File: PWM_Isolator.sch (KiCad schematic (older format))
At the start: 12 parts, among them P1 PWM_OUT_1, P10 PWM_OUT_2, P2 PWR_Jumper1, P3 Motor_Pwr1, P4 GND_IN_1, P5 Pololu PWM + Power rail, P6 NC, P7 GND_IN_2, P8 PWR_Jumper2, P9 Motor_Pwr2, U1 Si8660BA-B-IS1, U2 Si8660BA-B-IS1

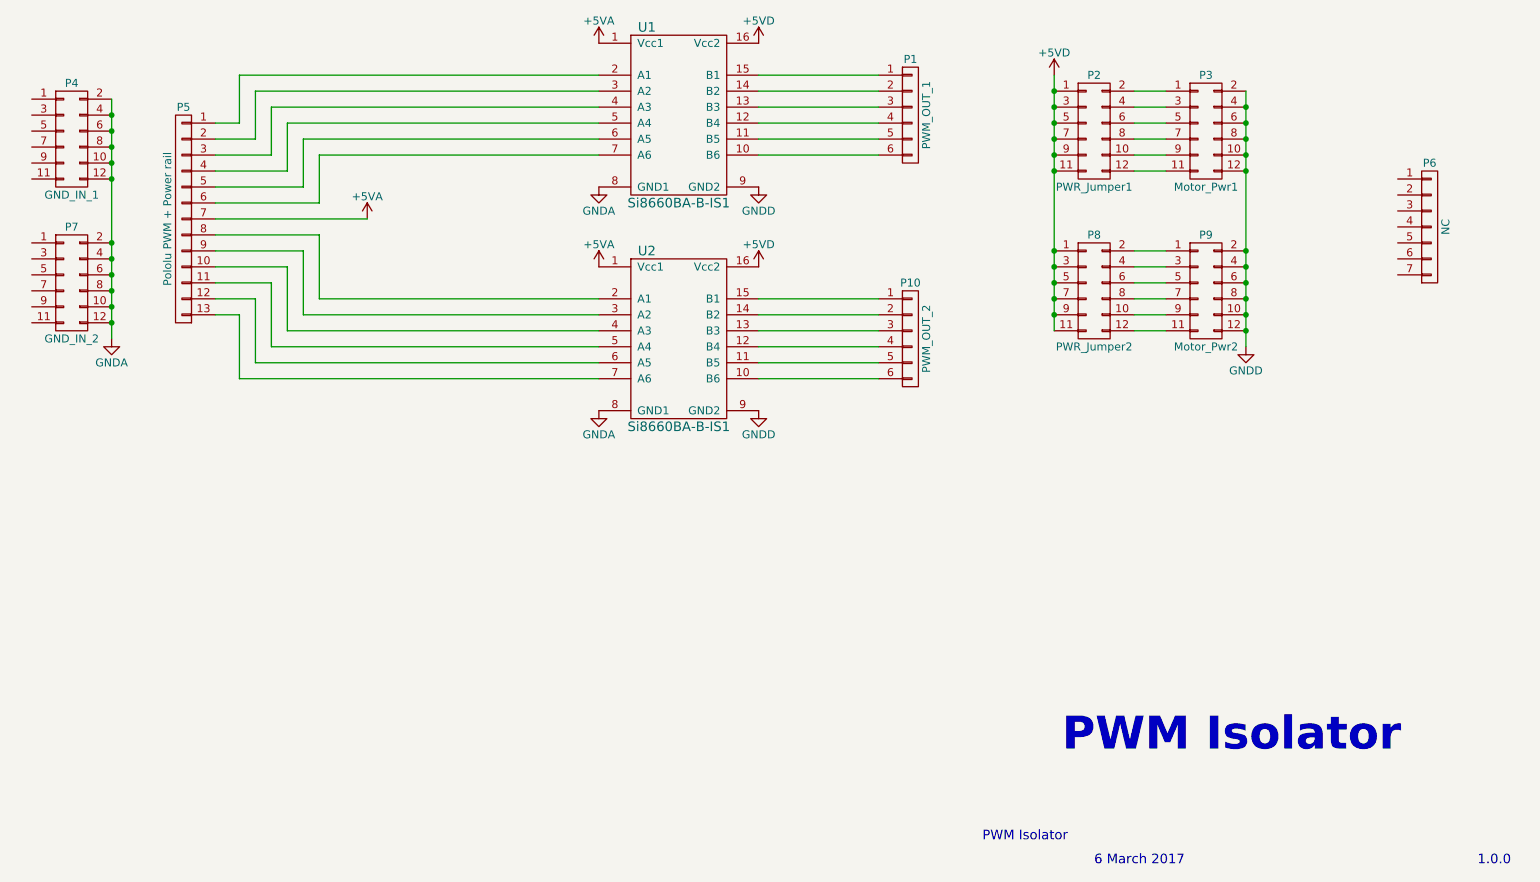
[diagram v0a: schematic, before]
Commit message: Finished with PCB and Net
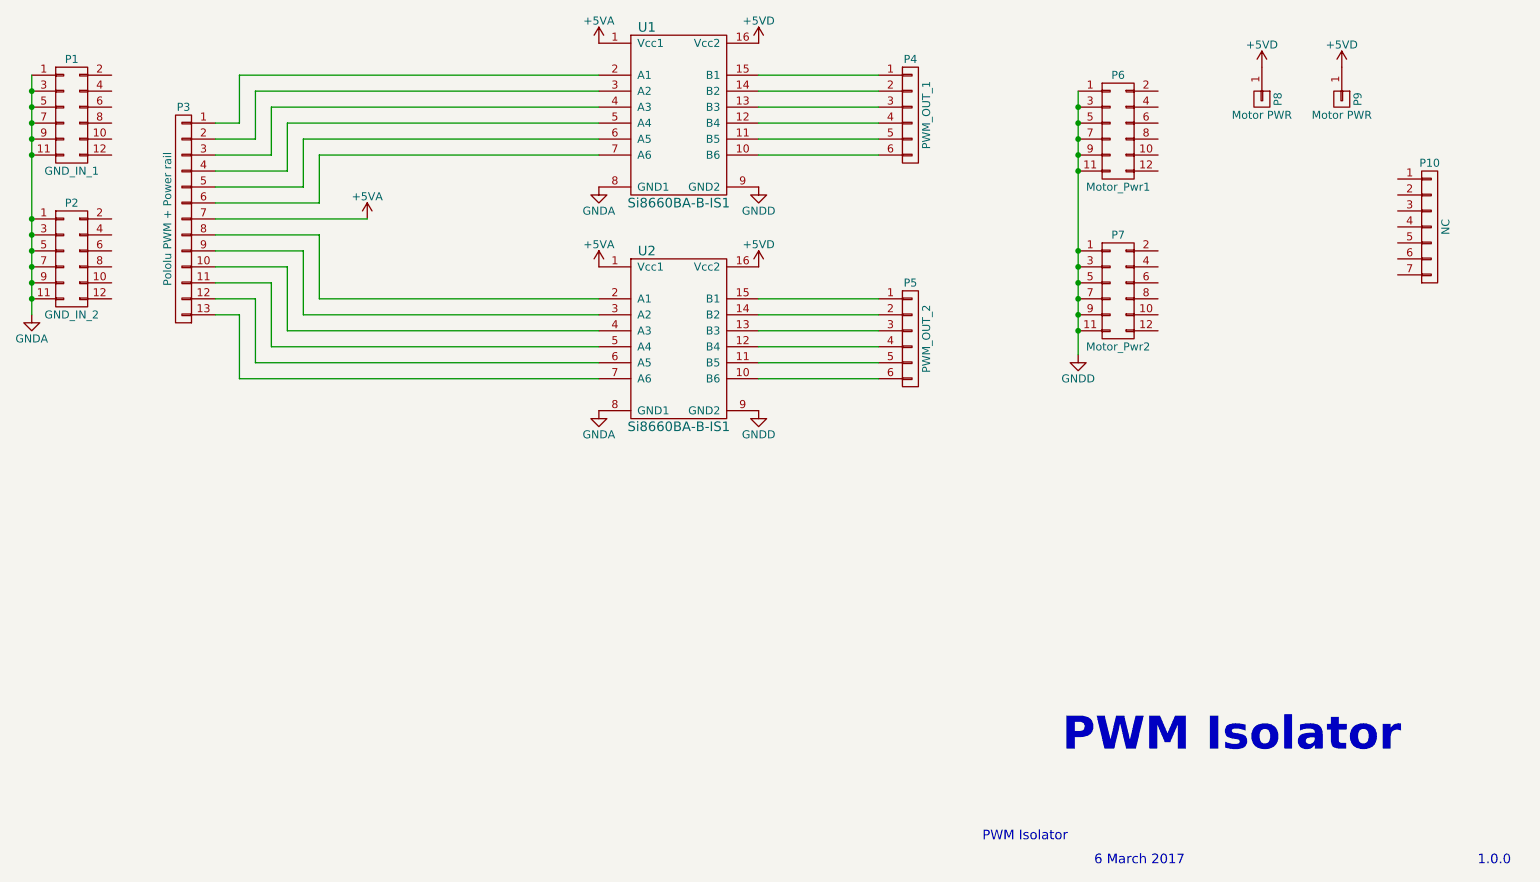
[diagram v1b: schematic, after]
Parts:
- removed P2: PWR_Jumper1, Pin_Headers:Pin_Header_Straight_SMT_02x06, symbol CONN_02X06
- removed P8: PWR_Jumper2, Pin_Headers:Pin_Header_Straight_SMT_02x06, symbol CONN_02X06
- added P8, P9: Motor PWR, Pin_Headers:Pin_Header_Straight_1x01, symbol CONN_01X01
- renumbered P4 to P1, P6 to P10, P7 to P2, P5 to P3, P1 to P4, P10 to P5, P3 to P6, P9 to P7
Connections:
- net +5VD: now also P8.1 (P1), P9.1 (P1)
- net GNDA: now also P1.1 (P1), P1.11 (P11), P1.3 (P3), P1.5 (P5), P1.7 (P7), P1.9 (P9), P2.1 (P1), P2.11 (P11), P2.3 (P3), P2.5 (P5), P2.7 (P7), P2.9 (P9); no longer P1.10 (P10), P1.12 (P12), P1.2 (P2), P1.4 (P4), P1.6 (P6), P1.8 (P8), P2.10 (P10), P2.12 (P12), P2.2 (P2), P2.4 (P4), P2.6 (P6), P2.8 (P8)
- net GNDD: now also P6.1 (P1), P6.11 (P11), P6.3 (P3), P6.5 (P5), P6.7 (P7), P6.9 (P9), P7.1 (P1), P7.11 (P11), P7.3 (P3), P7.5 (P5), P7.7 (P7), P7.9 (P9); no longer P6.10 (P10), P6.12 (P12), P6.2 (P2), P6.4 (P4), P6.6 (P6), P6.8 (P8), P7.10 (P10), P7.12 (P12), P7.2 (P2), P7.4 (P4), P7.6 (P6), P7.8 (P8)
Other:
- moved on the sheet: P1, P2, P6, P7
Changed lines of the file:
@@
 LIBS:valves
 LIBS:zeabus
+LIBS:PWM_Isolator-cache
 EELAYER 25 0
 EELAYER END
@@
 $EndComp
 $Comp
-L CONN_01X13 P5
+L CONN_01X13 P3
 U 1 1 58BD71B6
 P 2550 3600
-F 0 "P5" H 2550 4300 50  0000 C CNN
+F 0 "P3" H 2550 4300 50  0000 C CNN
 F 1 "Pololu PWM + Power rail" V 2650 3600 50  0000 C CNN
 F 2 "Socket_Strips:Socket_Strip_Straight_1x13" H 2550 3600 50  0001 C CNN
@@
 $EndComp
 $Comp
-L CONN_02X06 P7
+L CONN_02X06 P2
 U 1 1 58BD71DC
-P 1850 4000
-F 0 "P7" H 1850 4350 50  0000 C CNN
-F 1 "GND_IN_2" H 1850 3650 50  0000 C CNN
-F 2 "Socket_Strips:Socket_Strip_Straight_2x06" H 1850 2800 50  0001 C CNN
-F 3 "" H 1850 2800 50  0000 C CNN
-	1    1850 4000
-	1    0    0    -1
-$EndComp
-$Comp
-L CONN_01X07 P6
+P 1850 3850
+F 0 "P2" H 1850 4200 50  0000 C CNN
+F 1 "GND_IN_2" H 1850 3500 50  0000 C CNN
+F 2 "Socket_Strips:Socket_Strip_Straight_2x06" H 1850 2650 50  0001 C CNN
+F 3 "" H 1850 2650 50  0000 C CNN
+	1    1850 3850
+	1    0    0    -1
+$EndComp
+$Comp
+L CONN_01X07 P10
 U 1 1 58BD7246
 P 10350 3650
-F 0 "P6" H 10350 4050 50  0000 C CNN
+F 0 "P10" H 10350 4050 50  0000 C CNN
 F 1 "NC" V 10450 3650 50  0000 C CNN
 F 2 "Socket_Strips:Socket_Strip_Straight_1x07" H 10350 3650 50  0001 C CNN
@@
 $EndComp
 $Comp
-L CONN_02X06 P4
+L CONN_02X06 P1
 U 1 1 58BD72FA
-P 1850 3100
-F 0 "P4" H 1850 3450 50  0000 C CNN
-F 1 "GND_IN_1" H 1850 2750 50  0000 C CNN
-F 2 "Socket_Strips:Socket_Strip_Straight_2x06" H 1850 1900 50  0001 C CNN
-F 3 "" H 1850 1900 50  0000 C CNN
-	1    1850 3100
-	1    0    0    -1
-$EndComp
-$Comp
-L CONN_02X06 P3
+P 1850 2950
+F 0 "P1" H 1850 3300 50  0000 C CNN
+F 1 "GND_IN_1" H 1850 2600 50  0000 C CNN
+F 2 "Socket_Strips:Socket_Strip_Straight_2x06" H 1850 1750 50  0001 C CNN
+F 3 "" H 1850 1750 50  0000 C CNN
+	1    1850 2950
+	1    0    0    -1
+$EndComp
+$Comp
+L CONN_02X06 P6
 U 1 1 58BD7333
-P 8950 3050
-F 0 "P3" H 8950 3400 50  0000 C CNN
-F 1 "Motor_Pwr1" H 8950 2700 50  0000 C CNN
-F 2 "Pin_Headers:Pin_Header_Straight_2x06" H 8950 1850 50  0001 C CNN
-F 3 "" H 8950 1850 50  0000 C CNN
-	1    8950 3050
-	1    0    0    -1
-$EndComp
-$Comp
-L CONN_02X06 P2
-U 1 1 58BD7377
-P 8250 3050
-F 0 "P2" H 8250 3400 50  0000 C CNN
-F 1 "PWR_Jumper1" H 8250 2700 50  0000 C CNN
-F 2 "Pin_Headers:Pin_Header_Straight_SMT_02x06" H 8250 1850 50  0001 C CNN
-F 3 "" H 8250 1850 50  0000 C CNN
-	1    8250 3050
-	1    0    0    -1
-$EndComp
-$Comp
-L CONN_01X06 P1
+P 8400 3050
+F 0 "P6" H 8400 3400 50  0000 C CNN
+F 1 "Motor_Pwr1" H 8400 2700 50  0000 C CNN
+F 2 "Pin_Headers:Pin_Header_Straight_2x06" H 8400 1850 50  0001 C CNN
+F 3 "" H 8400 1850 50  0000 C CNN
+	1    8400 3050
+	1    0    0    -1
+$EndComp
+$Comp
+L CONN_01X06 P4
 U 1 1 58BD73C1
 P 7100 2950
-F 0 "P1" H 7100 3300 50  0000 C CNN
+F 0 "P4" H 7100 3300 50  0000 C CNN
 F 1 "PWM_OUT_1" V 7200 2950 50  0000 C CNN
 F 2 "Pin_Headers:Pin_Header_Straight_1x06" H 7100 2950 50  0001 C CNN
@@
 $EndComp
 $Comp
-L CONN_01X06 P10
+L CONN_01X06 P5
 U 1 1 58BD7462
 P 7100 4350
-F 0 "P10" H 7100 4700 50  0000 C CNN
+F 0 "P5" H 7100 4700 50  0000 C CNN
 F 1 "PWM_OUT_2" V 7200 4350 50  0000 C CNN
 F 2 "Pin_Headers:Pin_Header_Straight_1x06" H 7100 4350 50  0001 C CNN
@@
 $EndComp
 $Comp
-L CONN_02X06 P8
-U 1 1 58BD749E
-P 8250 4050
-F 0 "P8" H 8250 4400 50  0000 C CNN
-F 1 "PWR_Jumper2" H 8250 3700 50  0000 C CNN
-F 2 "Pin_Headers:Pin_Header_Straight_SMT_02x06" H 8250 2850 50  0001 C CNN
-F 3 "" H 8250 2850 50  0000 C CNN
-	1    8250 4050
-	1    0    0    -1
-$EndComp
-$Comp
-L CONN_02X06 P9
+L CONN_02X06 P7
 U 1 1 58BD7515
-P 8950 4050
-F 0 "P9" H 8950 4400 50  0000 C CNN
-F 1 "Motor_Pwr2" H 8950 3700 50  0000 C CNN
-F 2 "Pin_Headers:Pin_Header_Straight_2x06" H 8950 2850 50  0001 C CNN
-F 3 "" H 8950 2850 50  0000 C CNN
-	1    8950 4050
-	1    0    0    -1
-$EndComp
-Wire Wire Line
-	2100 2850 2100 4350
-Connection ~ 2100 2950
-Connection ~ 2100 3050
-Connection ~ 2100 3150
-Connection ~ 2100 3250
-Connection ~ 2100 3350
-Connection ~ 2100 3750
-Connection ~ 2100 3850
-Connection ~ 2100 3950
-Connection ~ 2100 4050
-Connection ~ 2100 4150
+P 8400 4050
+F 0 "P7" H 8400 4400 50  0000 C CNN
+F 1 "Motor_Pwr2" H 8400 3700 50  0000 C CNN
+F 2 "Pin_Headers:Pin_Header_Straight_2x06" H 8400 2850 50  0001 C CNN
+F 3 "" H 8400 2850 50  0000 C CNN
+	1    8400 4050
+	1    0    0    -1
+$EndComp
 $Comp
 L GNDA #PWR01
 U 1 1 58BD7AF0
-P 2100 4350
-F 0 "#PWR01" H 2100 4100 50  0001 C CNN
-F 1 "GNDA" H 2100 4200 50  0000 C CNN
-F 2 "" H 2100 4350 50  0000 C CNN
-F 3 "" H 2100 4350 50  0000 C CNN
-	1    2100 4350
+P 1600 4200
+F 0 "#PWR01" H 1600 3950 50  0001 C CNN
+F 1 "GNDA" H 1600 4050 50  0000 C CNN
+F 2 "" H 1600 4200 50  0000 C CNN
+F 3 "" H 1600 4200 50  0000 C CNN
+	1    1600 4200
 	1    0    0    -1
 $EndComp
@@
 	1    0    0    -1
 $EndComp
-Connection ~ 2100 4250
 Wire Wire Line
 	2750 3000 2900 3000
@@
 L +5VD #PWR04
 U 1 1 58BD81D8
-P 8000 2700
-F 0 "#PWR04" H 8000 2550 50  0001 C CNN
-F 1 "+5VD" H 8000 2840 50  0000 C CNN
-F 2 "" H 8000 2700 50  0000 C CNN
-F 3 "" H 8000 2700 50  0000 C CNN
-	1    8000 2700
+P 9300 2650
+F 0 "#PWR04" H 9300 2500 50  0001 C CNN
+F 1 "+5VD" H 9300 2790 50  0000 C CNN
+F 2 "" H 9300 2650 50  0000 C CNN
+F 3 "" H 9300 2650 50  0000 C CNN
+	1    9300 2650
 	1    0    0    -1
 $EndComp
@@
 Wire Wire Line
 	6150 4600 6900 4600
-Wire Wire Line
-	8500 2800 8700 2800
-Wire Wire Line
-	8700 2900 8500 2900
-Wire Wire Line
-	8500 3000 8700 3000
-Wire Wire Line
-	8700 3100 8500 3100
-Wire Wire Line
-	8500 3200 8700 3200
-Wire Wire Line
-	8700 3300 8500 3300
-Wire Wire Line
-	8500 3800 8700 3800
-Wire Wire Line
-	8700 3900 8500 3900
-Wire Wire Line
-	8700 4000 8500 4000
-Wire Wire Line
-	8500 4100 8700 4100
-Wire Wire Line
-	8700 4200 8500 4200
-Wire Wire Line
-	8500 4300 8700 4300
-Wire Wire Line
-	9200 2800 9200 4400
-Connection ~ 9200 4200
-Connection ~ 9200 4100
-Connection ~ 9200 4000
-Connection ~ 9200 3900
-Connection ~ 9200 3800
-Connection ~ 9200 3300
-Connection ~ 9200 3200
-Connection ~ 9200 3100
-Connection ~ 9200 3000
-Connection ~ 9200 2900
 $Comp
 L GNDD #PWR07
 U 1 1 58BD98A2
-P 9200 4400
-F 0 "#PWR07" H 9200 4150 50  0001 C CNN
-F 1 "GNDD" H 9200 4250 50  0000 C CNN
-F 2 "" H 9200 4400 50  0000 C CNN
-F 3 "" H 9200 4400 50  0000 C CNN
-	1    9200 4400
+P 8150 4450
+F 0 "#PWR07" H 8150 4200 50  0001 C CNN
+F 1 "GNDD" H 8150 4300 50  0000 C CNN
+F 2 "" H 8150 4450 50  0000 C CNN
+F 3 "" H 8150 4450 50  0000 C CNN
+	1    8150 4450
 	1    0    0    -1
 $EndComp
@@
 	1    0    0    -1
 $EndComp
-Connection ~ 9200 4300
-Wire Wire Line
-	8000 2700 8000 4300
-Connection ~ 8000 4200
-Connection ~ 8000 4100
-Connection ~ 8000 4000
-Connection ~ 8000 3900
-Connection ~ 8000 3800
-Connection ~ 8000 3300
-Connection ~ 8000 3200
-Connection ~ 8000 3100
-Connection ~ 8000 3000
-Connection ~ 8000 2900
 $Comp
 L +5VA #PWR010
@@
 	1    0    0    -1
 $EndComp
-Connection ~ 8000 2800
 Text Notes 8050 6950 0    206  ~ 41
 PWM Isolator\n
@@
 Text Notes 7550 7500 0    60   ~ 0
 PWM Isolator\n
+Wire Wire Line
+	1600 2700 1600 4200
+Connection ~ 1600 2800
+Connection ~ 1600 2900
+Connection ~ 1600 3000
+Connection ~ 1600 3100
+Connection ~ 1600 3200
+Connection ~ 1600 3600
+Connection ~ 1600 3700
+Connection ~ 1600 3800
+Connection ~ 1600 3900
+Connection ~ 1600 4000
+Connection ~ 1600 4100
+Wire Wire Line
+	8150 2800 8150 4450
+Connection ~ 8150 2900
+Connection ~ 8150 3000
+Connection ~ 8150 3100
+Connection ~ 8150 3200
+Connection ~ 8150 3300
+Connection ~ 8150 3800
+Connection ~ 8150 3900
+Connection ~ 8150 4000
+Connection ~ 8150 4100
+Connection ~ 8150 4200
+Connection ~ 8150 4300
+$Comp
+L CONN_01X01 P8
+U 1 1 58BE358F
+P 9300 2850
+F 0 "P8" H 9300 2950 50  0000 C CNN
+F 1 "Motor PWR" V 9400 2850 50  0000 C CNN
+F 2 "Pin_Headers:Pin_Header_Straight_1x01" H 9300 2850 50  0001 C CNN
+F 3 "" H 9300 2850 50  0000 C CNN
+	1    9300 2850
+	0    1    1    0
+$EndComp
+$Comp
+L +5VD #PWR?
+U 1 1 58BE3A9C
+P 9800 2650
+F 0 "#PWR?" H 9800 2500 50  0001 C CNN
+F 1 "+5VD" H 9800 2790 50  0000 C CNN
+F 2 "" H 9800 2650 50  0000 C CNN
+F 3 "" H 9800 2650 50  0000 C CNN
+	1    9800 2650
+	1    0    0    -1
+$EndComp
+$Comp
+L CONN_01X01 P9
+U 1 1 58BE3AA2
+P 9800 2850
+F 0 "P9" H 9800 2950 50  0000 C CNN
+F 1 "Motor PWR" V 9900 2850 50  0000 C CNN
+F 2 "Pin_Headers:Pin_Header_Straight_1x01" H 9800 2850 50  0001 C CNN
+F 3 "" H 9800 2850 50  0000 C CNN
+	1    9800 2850
+	0    1    1    0
+$EndComp
 $EndSCHEMATC

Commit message: Change footprint of Si8660 and re-route the PCB.
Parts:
- U1, U2: footprint SMD_Packages:SO-16-N -> Zeabus:Narrow-SOIC-16
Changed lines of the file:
@@
 F 0 "U1" H 5450 2600 60  0000 C CNN
 F 1 "Si8660BA-B-IS1" H 5650 1500 60  0000 C CNN
-F 2 "SMD_Packages:SO-16-N" H 5150 2500 60  0001 C CNN
+F 2 "Zeabus:Narrow-SOIC-16" H 5150 2500 60  0001 C CNN
 F 3 "" H 5150 2500 60  0001 C CNN
 	1    5150 2500
@@
 F 0 "U2" H 5450 4000 60  0000 C CNN
 F 1 "Si8660BA-B-IS1" H 5650 2900 60  0000 C CNN
-F 2 "SMD_Packages:SO-16-N" H 5150 3900 60  0001 C CNN
+F 2 "Zeabus:Narrow-SOIC-16" H 5150 3900 60  0001 C CNN
 F 3 "" H 5150 3900 60  0001 C CNN
 	1    5150 3900
@@
 $EndComp
 $Comp
-L +5VD #PWR?
+L +5VD #PWR013
 U 1 1 58BE3A9C
 P 9800 2650
-F 0 "#PWR?" H 9800 2500 50  0001 C CNN
+F 0 "#PWR013" H 9800 2500 50  0001 C CNN
 F 1 "+5VD" H 9800 2790 50  0000 C CNN
 F 2 "" H 9800 2650 50  0000 C CNN
